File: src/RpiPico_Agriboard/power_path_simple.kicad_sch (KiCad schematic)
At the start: 7 parts, among them Q12 BSP170P-VB, Q13 BSP170P-VB

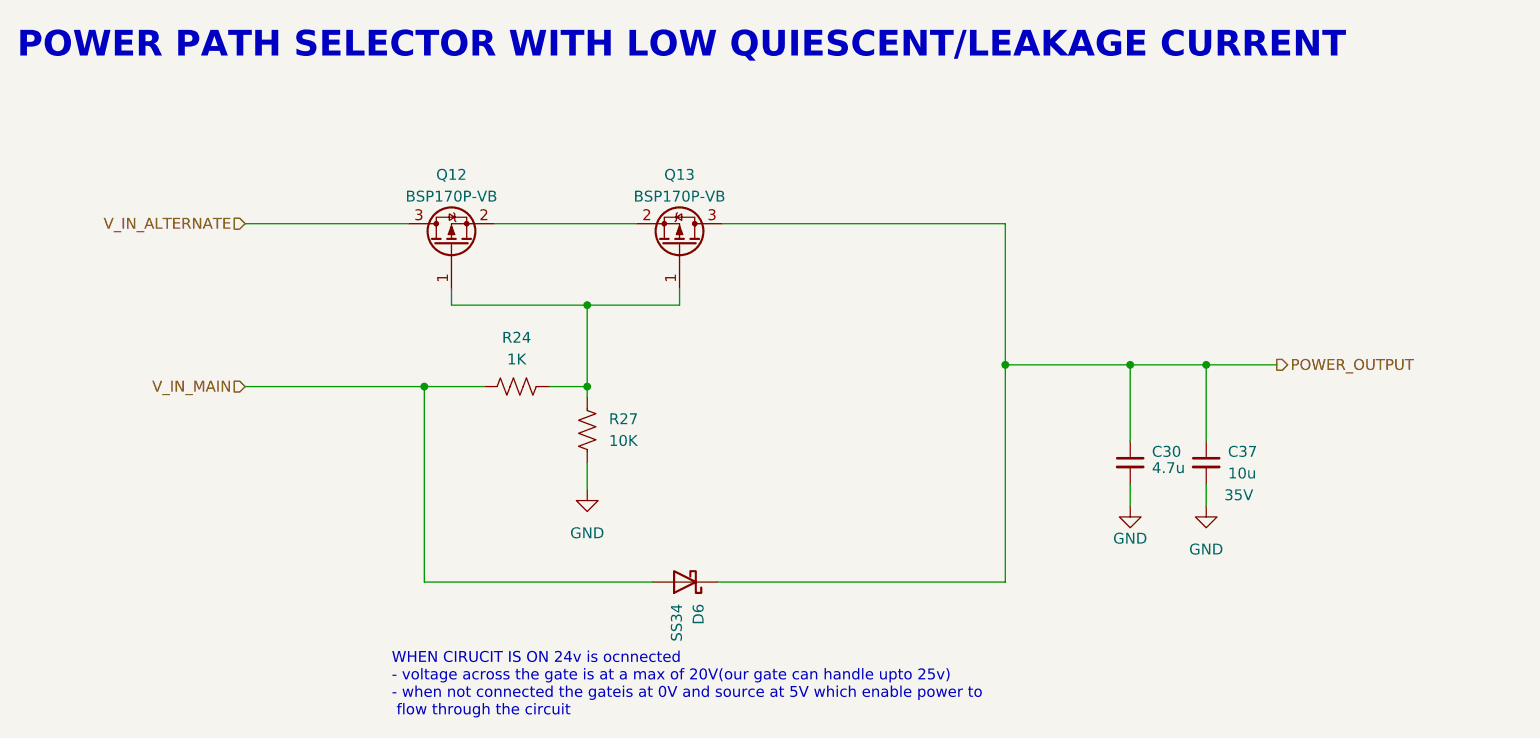
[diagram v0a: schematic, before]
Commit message: schematic updates completed
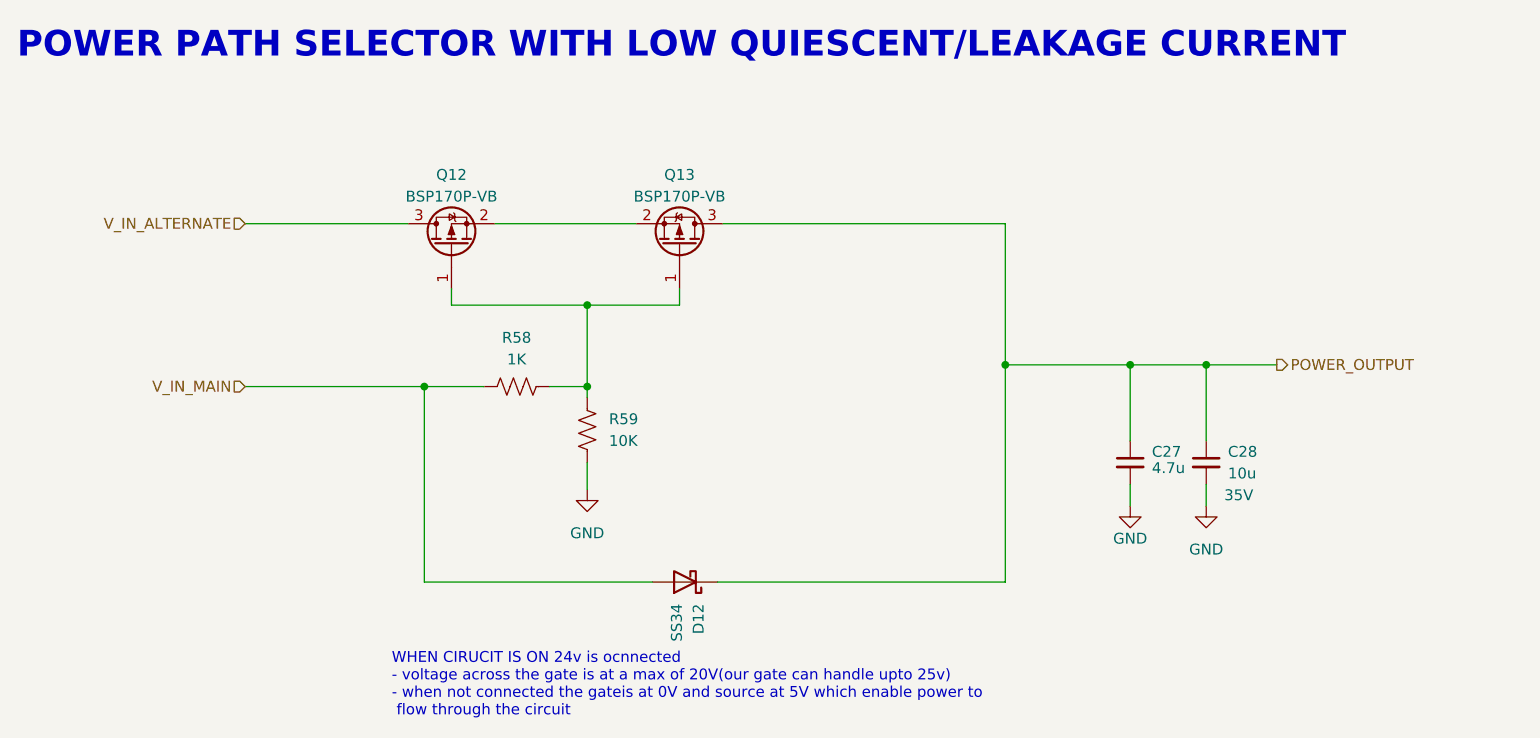
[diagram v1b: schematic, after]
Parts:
- renumbered C30 to C27, C37 to C28, D6 to D12, R24 to R58, R27 to R59
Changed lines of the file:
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@@
       )
       (project "RpiPico_Agriboard"
-        (path "/c2474b65-c0e8-4987-86b2-fddddd4113dc/6578793a-18cf-4100-aa8d-b3f918b44a8b/705d5845-37bb-48c7-9641-198316a19ba9"
-          (reference "Q12") (unit 1)
+        (path "/c2474b65-c0e8-4987-86b2-fddddd4113dc/f3a00526-8108-483c-9ec5-d5fcf6fe065b/e1b77c03-2b38-43f3-998b-3c2f1972d847"
+          (reference "Q?") (unit 1)
         )
       )
@@
   (symbol (lib_id "Device:C_Small") (at 206.375 102.87 0) (unit 1)
     (in_bom yes) (on_board yes) (dnp no)
-    (property "Reference" "C30" (at 208.915 101.6062 0)
+    (property "Reference" "C27" (at 208.915 101.6062 0)
       (effects (font (size 1.27 1.27)) (justify left))
     )
@@
       )
       (project "RpiPico_Agriboard"
-        (path "/c2474b65-c0e8-4987-86b2-fddddd4113dc/6578793a-18cf-4100-aa8d-b3f918b44a8b/705d5845-37bb-48c7-9641-198316a19ba9"
-          (reference "C30") (unit 1)
+        (path "/c2474b65-c0e8-4987-86b2-fddddd4113dc/f3a00526-8108-483c-9ec5-d5fcf6fe065b/e1b77c03-2b38-43f3-998b-3c2f1972d847"
+          (reference "C?") (unit 1)
         )
       )
@@
   (symbol (lib_id "Device:D_Schottky") (at 154.305 116.84 180) (unit 1)
     (in_bom yes) (on_board yes) (dnp no) (fields_autoplaced)
-    (property "Reference" "D6" (at 155.8926 119.38 90)
+    (property "Reference" "D12" (at 155.8926 119.38 90)
       (effects (font (size 1.27 1.27)) (justify left))
     )
@@
       )
       (project "RpiPico_Agriboard"
-        (path "/c2474b65-c0e8-4987-86b2-fddddd4113dc/6578793a-18cf-4100-aa8d-b3f918b44a8b/705d5845-37bb-48c7-9641-198316a19ba9"
-          (reference "D6") (unit 1)
+        (path "/c2474b65-c0e8-4987-86b2-fddddd4113dc/f3a00526-8108-483c-9ec5-d5fcf6fe065b/e1b77c03-2b38-43f3-998b-3c2f1972d847"
+          (reference "D?") (unit 1)
         )
       )
@@
       )
       (project "RpiPico_Agriboard"
-        (path "/c2474b65-c0e8-4987-86b2-fddddd4113dc/6578793a-18cf-4100-aa8d-b3f918b44a8b/705d5845-37bb-48c7-9641-198316a19ba9"
-          (reference "#PWR078") (unit 1)
+        (path "/c2474b65-c0e8-4987-86b2-fddddd4113dc/f3a00526-8108-483c-9ec5-d5fcf6fe065b/e1b77c03-2b38-43f3-998b-3c2f1972d847"
+          (reference "#PWR058") (unit 1)
         )
       )
@@
       )
       (project "RpiPico_Agriboard"
-        (path "/c2474b65-c0e8-4987-86b2-fddddd4113dc/6578793a-18cf-4100-aa8d-b3f918b44a8b/705d5845-37bb-48c7-9641-198316a19ba9"
-          (reference "#PWR080") (unit 1)
+        (path "/c2474b65-c0e8-4987-86b2-fddddd4113dc/f3a00526-8108-483c-9ec5-d5fcf6fe065b/e1b77c03-2b38-43f3-998b-3c2f1972d847"
+          (reference "#PWR060") (unit 1)
         )
       )
@@
   (symbol (lib_id "Device:R_US") (at 134.62 93.98 90) (unit 1)
     (in_bom yes) (on_board yes) (dnp no) (fields_autoplaced)
-    (property "Reference" "R24" (at 134.62 88.265 90)
+    (property "Reference" "R58" (at 134.62 88.265 90)
       (effects (font (size 1.27 1.27)))
     )
@@
       )
       (project "RpiPico_Agriboard"
-        (path "/c2474b65-c0e8-4987-86b2-fddddd4113dc/6578793a-18cf-4100-aa8d-b3f918b44a8b/705d5845-37bb-48c7-9641-198316a19ba9"
-          (reference "R24") (unit 1)
+        (path "/c2474b65-c0e8-4987-86b2-fddddd4113dc/f3a00526-8108-483c-9ec5-d5fcf6fe065b/e1b77c03-2b38-43f3-998b-3c2f1972d847"
+          (reference "R?") (unit 1)
         )
       )
@@
       )
       (project "RpiPico_Agriboard"
-        (path "/c2474b65-c0e8-4987-86b2-fddddd4113dc/6578793a-18cf-4100-aa8d-b3f918b44a8b/705d5845-37bb-48c7-9641-198316a19ba9"
-          (reference "#PWR079") (unit 1)
+        (path "/c2474b65-c0e8-4987-86b2-fddddd4113dc/f3a00526-8108-483c-9ec5-d5fcf6fe065b/e1b77c03-2b38-43f3-998b-3c2f1972d847"
+          (reference "#PWR059") (unit 1)
         )
       )
@@
       )
       (project "RpiPico_Agriboard"
-        (path "/c2474b65-c0e8-4987-86b2-fddddd4113dc/6578793a-18cf-4100-aa8d-b3f918b44a8b/705d5845-37bb-48c7-9641-198316a19ba9"
-          (reference "Q13") (unit 1)
+        (path "/c2474b65-c0e8-4987-86b2-fddddd4113dc/f3a00526-8108-483c-9ec5-d5fcf6fe065b/e1b77c03-2b38-43f3-998b-3c2f1972d847"
+          (reference "Q?") (unit 1)
         )
       )
@@
   (symbol (lib_id "Device:R_US") (at 142.875 99.06 0) (unit 1)
     (in_bom yes) (on_board yes) (dnp no) (fields_autoplaced)
-    (property "Reference" "R27" (at 145.415 97.7899 0)
+    (property "Reference" "R59" (at 145.415 97.7899 0)
       (effects (font (size 1.27 1.27)) (justify left))
     )
@@
       )
       (project "RpiPico_Agriboard"
-        (path "/c2474b65-c0e8-4987-86b2-fddddd4113dc/6578793a-18cf-4100-aa8d-b3f918b44a8b/705d5845-37bb-48c7-9641-198316a19ba9"
-          (reference "R27") (unit 1)
+        (path "/c2474b65-c0e8-4987-86b2-fddddd4113dc/f3a00526-8108-483c-9ec5-d5fcf6fe065b/e1b77c03-2b38-43f3-998b-3c2f1972d847"
+          (reference "R?") (unit 1)
         )
       )
@@
   (symbol (lib_id "Device:C_Small") (at 215.265 102.87 0) (unit 1)
     (in_bom yes) (on_board yes) (dnp no)
-    (property "Reference" "C37" (at 217.805 101.6062 0)
+    (property "Reference" "C28" (at 217.805 101.6062 0)
       (effects (font (size 1.27 1.27)) (justify left))
     )
@@
       )
       (project "RpiPico_Agriboard"
-        (path "/c2474b65-c0e8-4987-86b2-fddddd4113dc/6578793a-18cf-4100-aa8d-b3f918b44a8b/705d5845-37bb-48c7-9641-198316a19ba9"
-          (reference "C37") (unit 1)
-        )
-      )
+        (path "/c2474b65-c0e8-4987-86b2-fddddd4113dc/f3a00526-8108-483c-9ec5-d5fcf6fe065b/e1b77c03-2b38-43f3-998b-3c2f1972d847"
+          (reference "C?") (unit 1)
+        )
+      )
